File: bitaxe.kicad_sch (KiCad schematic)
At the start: 92 parts, among them IC1 BM1387, IC2 BM1387, IC3 MIC5317, IC4 MIC5317, J2 Conn_01x02, J3 Conn_01x05, J4 Conn_01x02, J5 Conn_01x03, Y1 25MHz

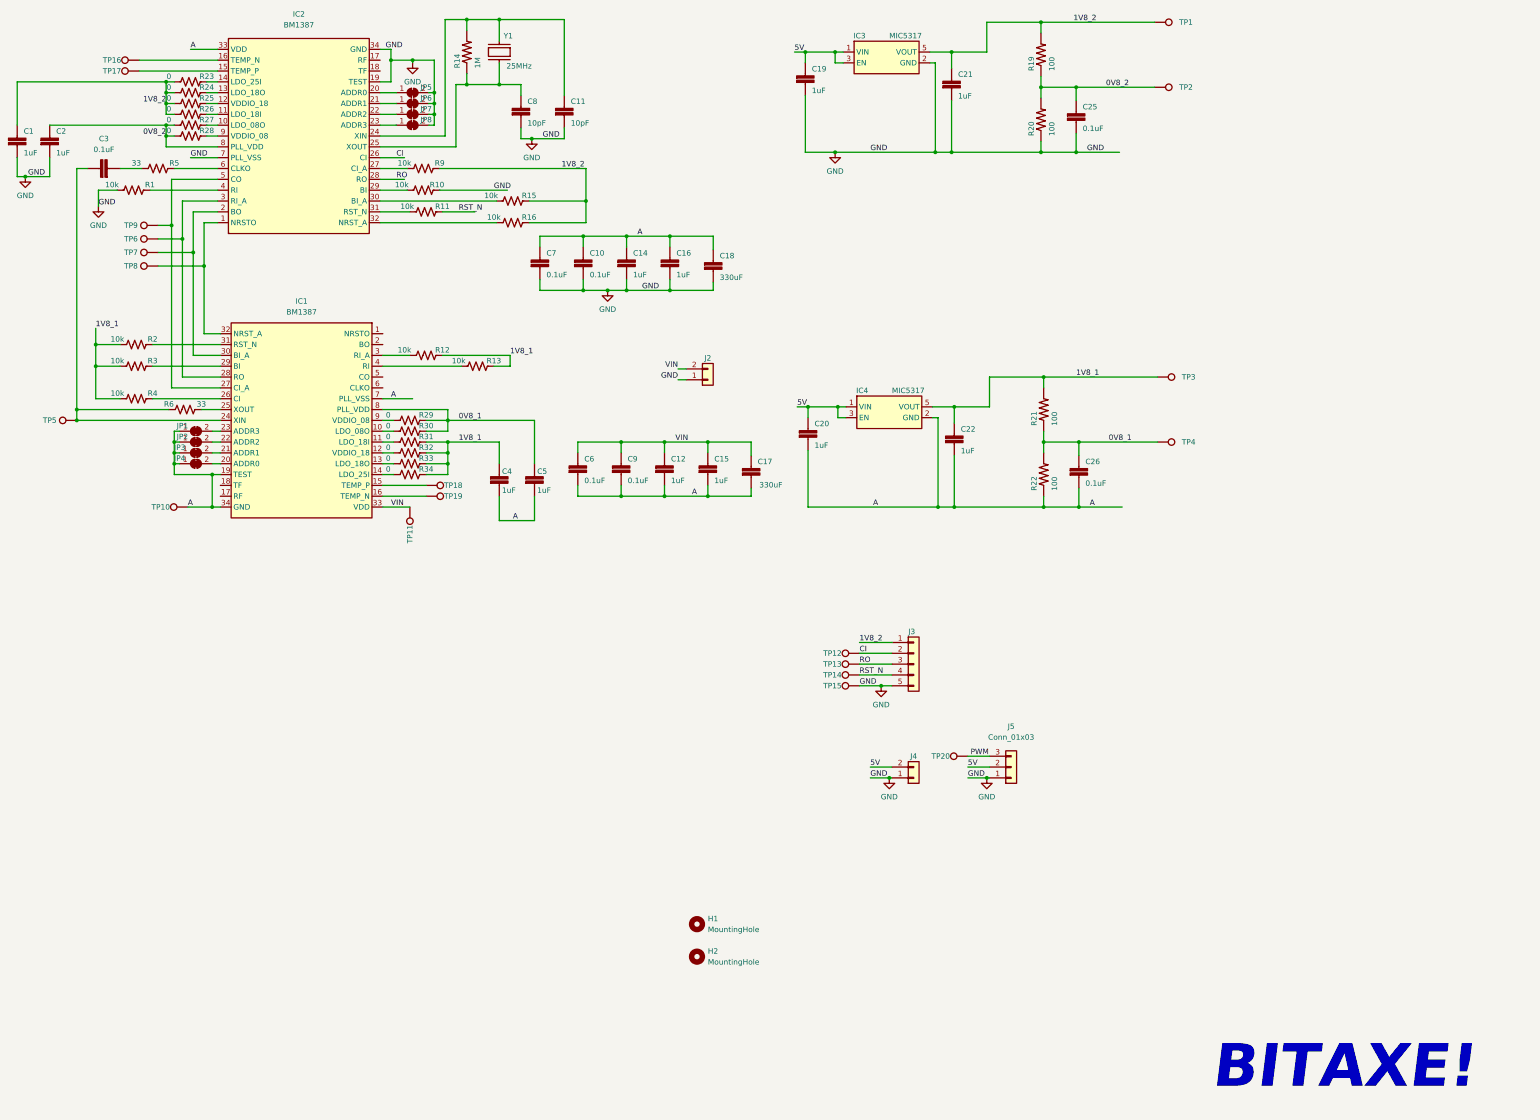
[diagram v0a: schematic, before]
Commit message: updated BOM and manufacturing files
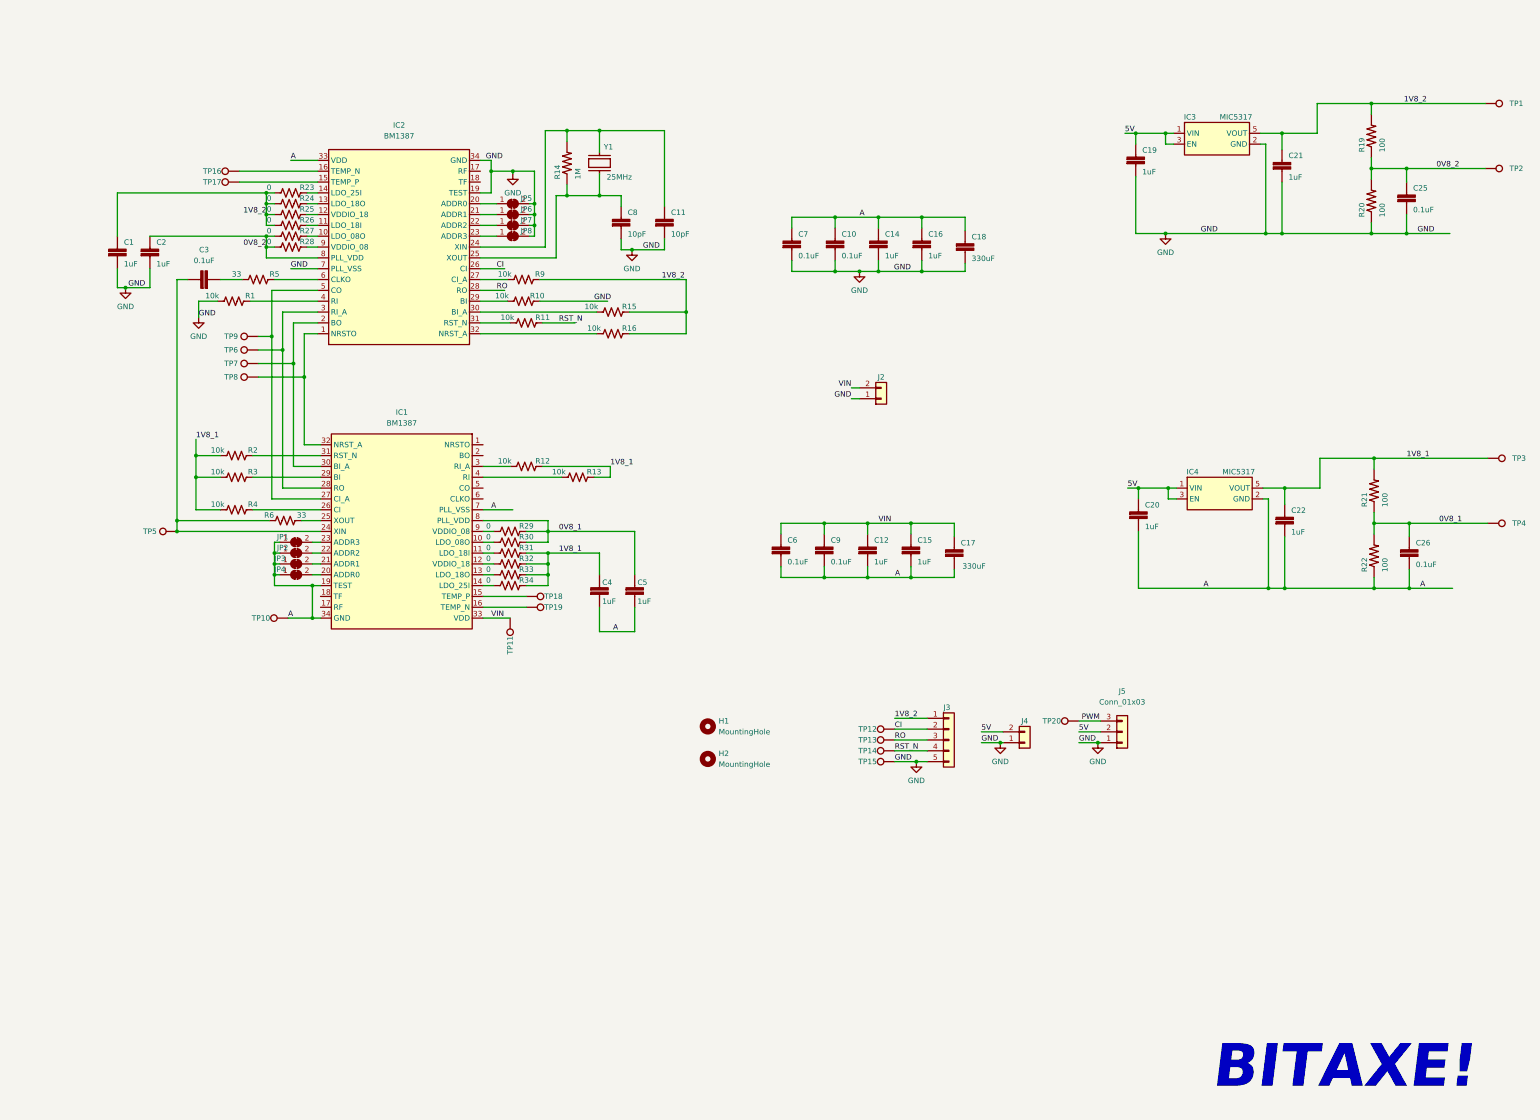
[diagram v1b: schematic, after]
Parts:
- C17, C18: DK 2388-PCT330/10DM-ND -> TCJD337M010R0025
- C3: DK (none) -> 1292-1639-1-ND
- H1, H2, JP1, JP2, JP3, JP4, JP5, JP6, JP7, JP8: DNP (none) -> T
- R1, R10, R11, R12, R13, R15, R16, R2, R3, R4, R9: DK (none) -> RMCF0402FT10K0CT-ND
- R22: DK RMCF0402FT10K0CT-ND -> RMCF0402FT12K4CT-ND
- R23, R24, R25, R26, R27, R28, R29, R30, R31, R32, R33, R34: DK (none) -> RMCF0402ZT0R00CT-ND
- R5, R6: DK (none) -> 311-33.0LRCT-ND
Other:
- moved on the sheet: C1, C10, C11, C12, C14, C15, C16, C17, C18, C19, C2, C20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
